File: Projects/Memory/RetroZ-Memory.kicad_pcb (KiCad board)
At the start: 2 copper layers, 100 x 80 mm, 21 parts, among them J1 Client Bus, U1 74LS32, U2 AT28C64B-15PU, U3 74LS138, U4 74HCT04, U5 74LS08, U6 AS6C4008-55PCN, U7 74HC273, U8 74LS08, U9 74LS138

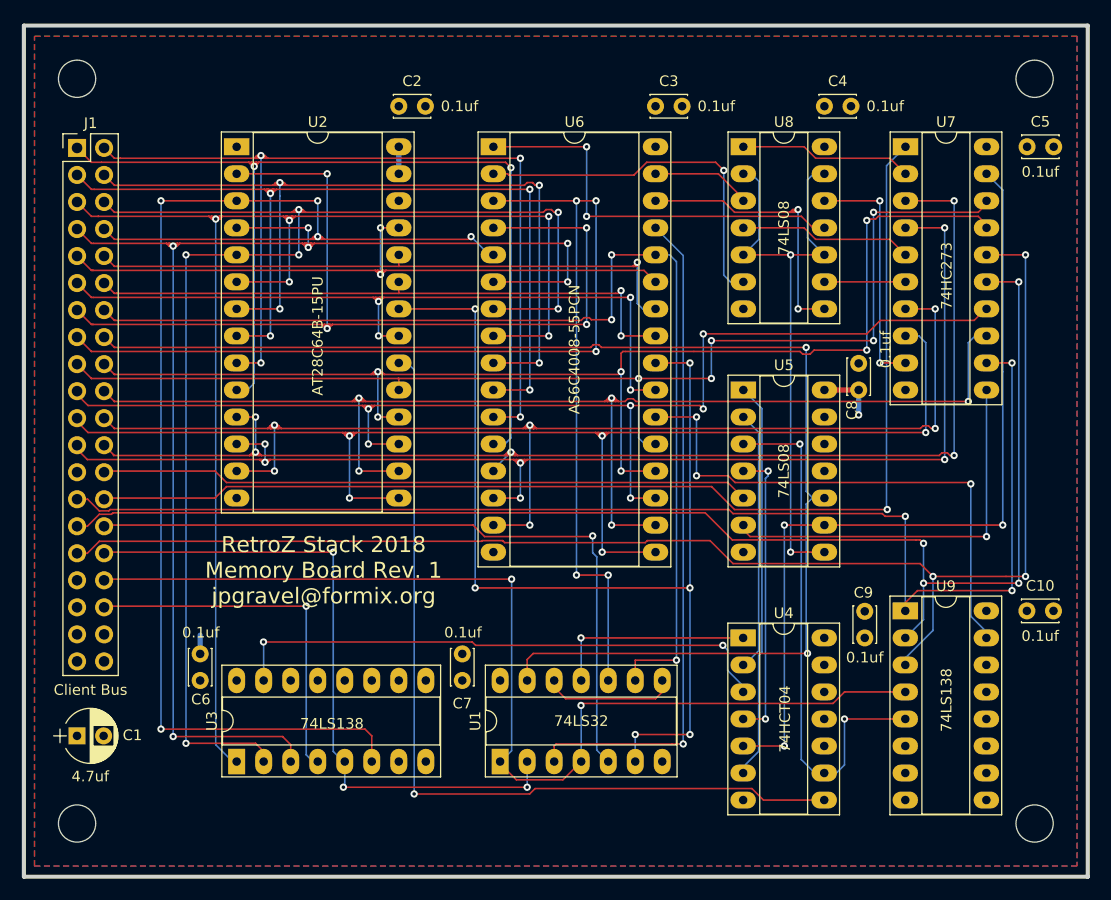
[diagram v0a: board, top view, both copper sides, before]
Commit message: finished sio2 board
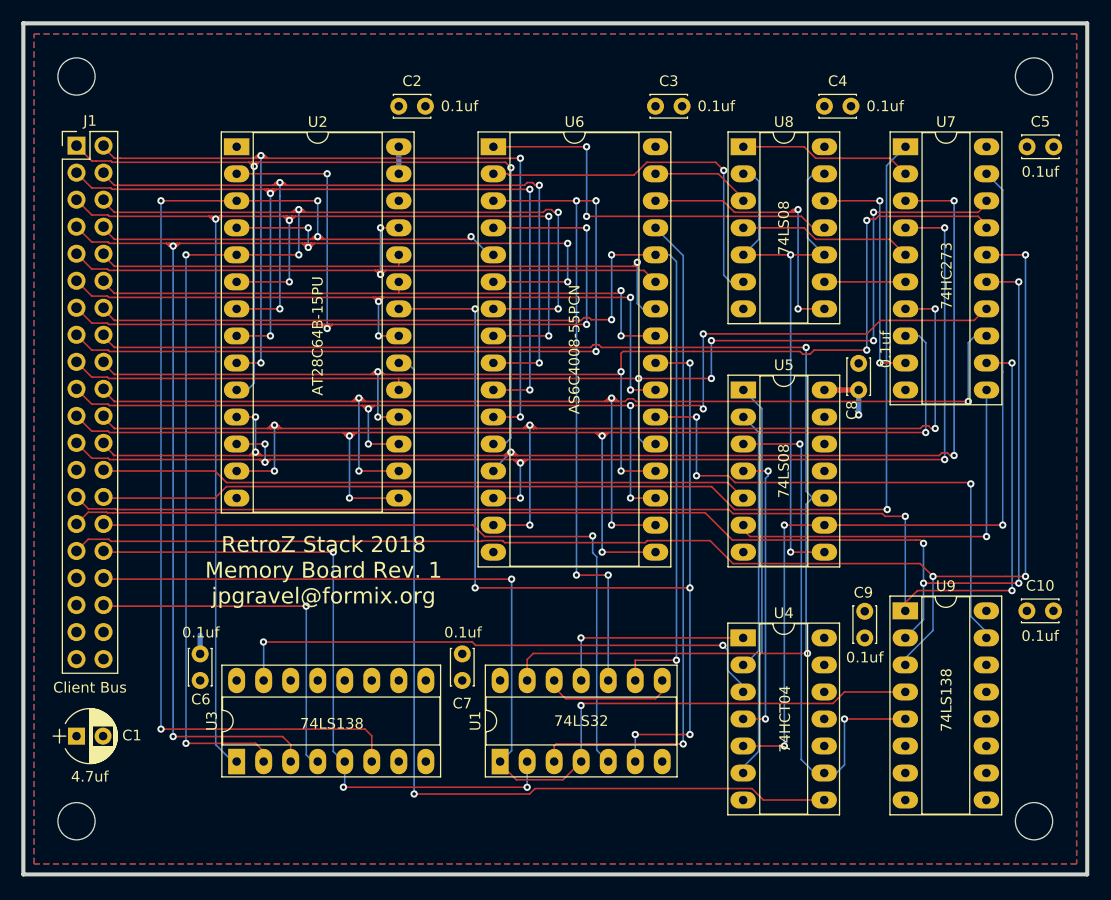
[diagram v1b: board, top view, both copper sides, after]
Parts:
- moved J1 0.22 mm to (94.9, 68.3)
- moved REF** 0.22 mm to (89.9, 136.8)
- moved C1 0.05 mm to (94.9, 123.8)
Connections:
- net A19 renamed DMA0
- net A20 renamed DMA1
- net A21 renamed DMA2
